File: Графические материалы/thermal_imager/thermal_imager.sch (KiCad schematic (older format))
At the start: 21 parts, among them J1 CONN_in-, J2 CONN_in+, J3 conOut+, J4 conOut-, J5 CONN_bat+, J6 CONN_bat-

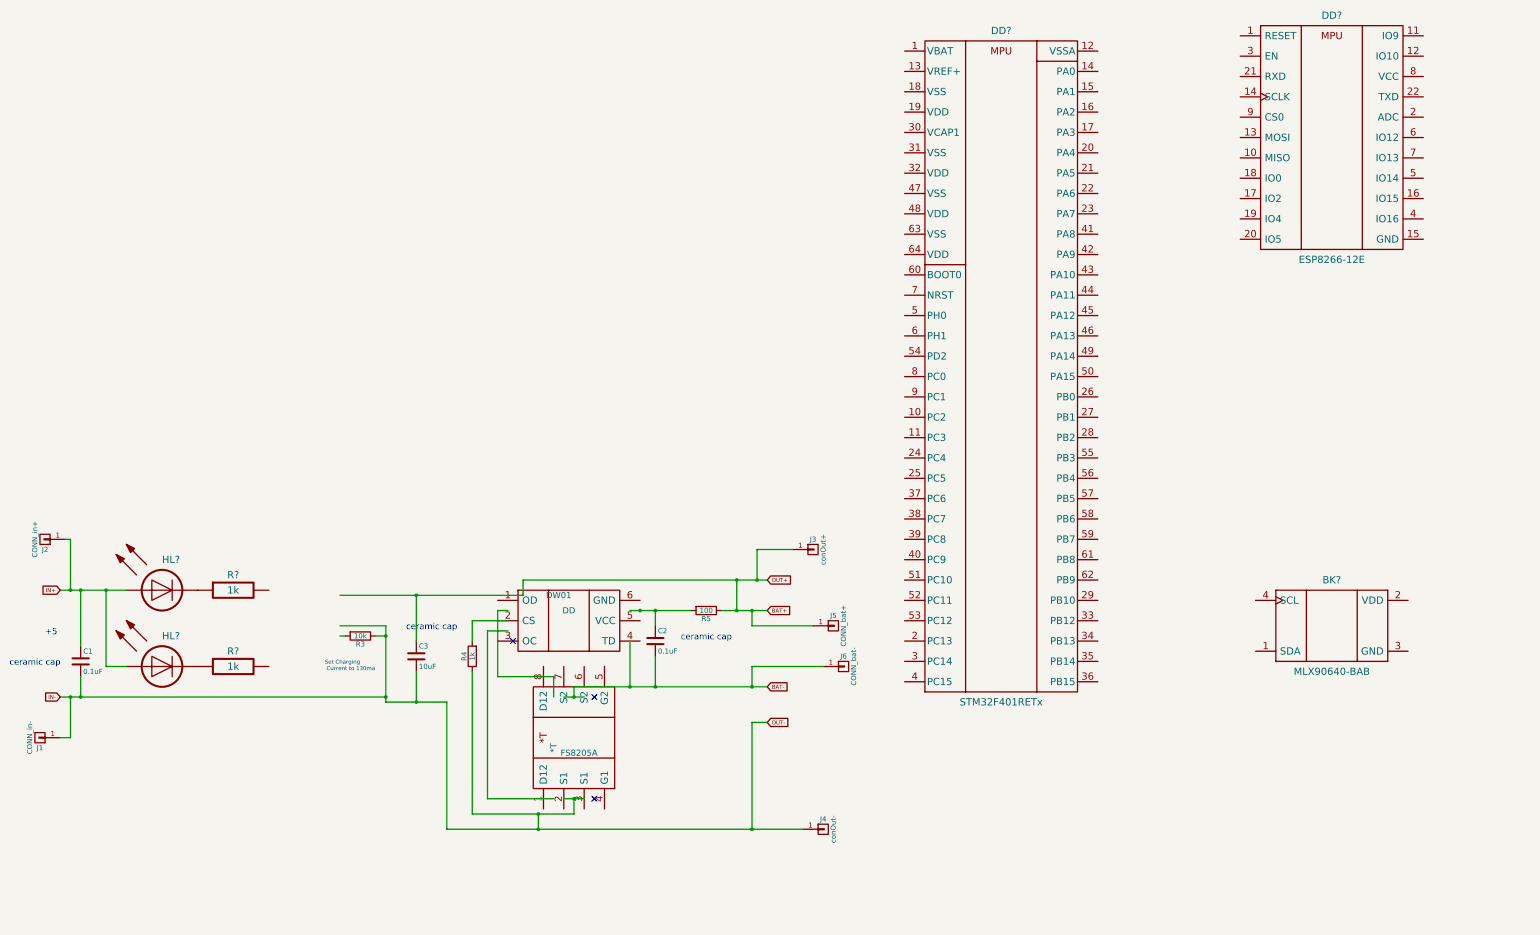
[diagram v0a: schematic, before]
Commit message: Something
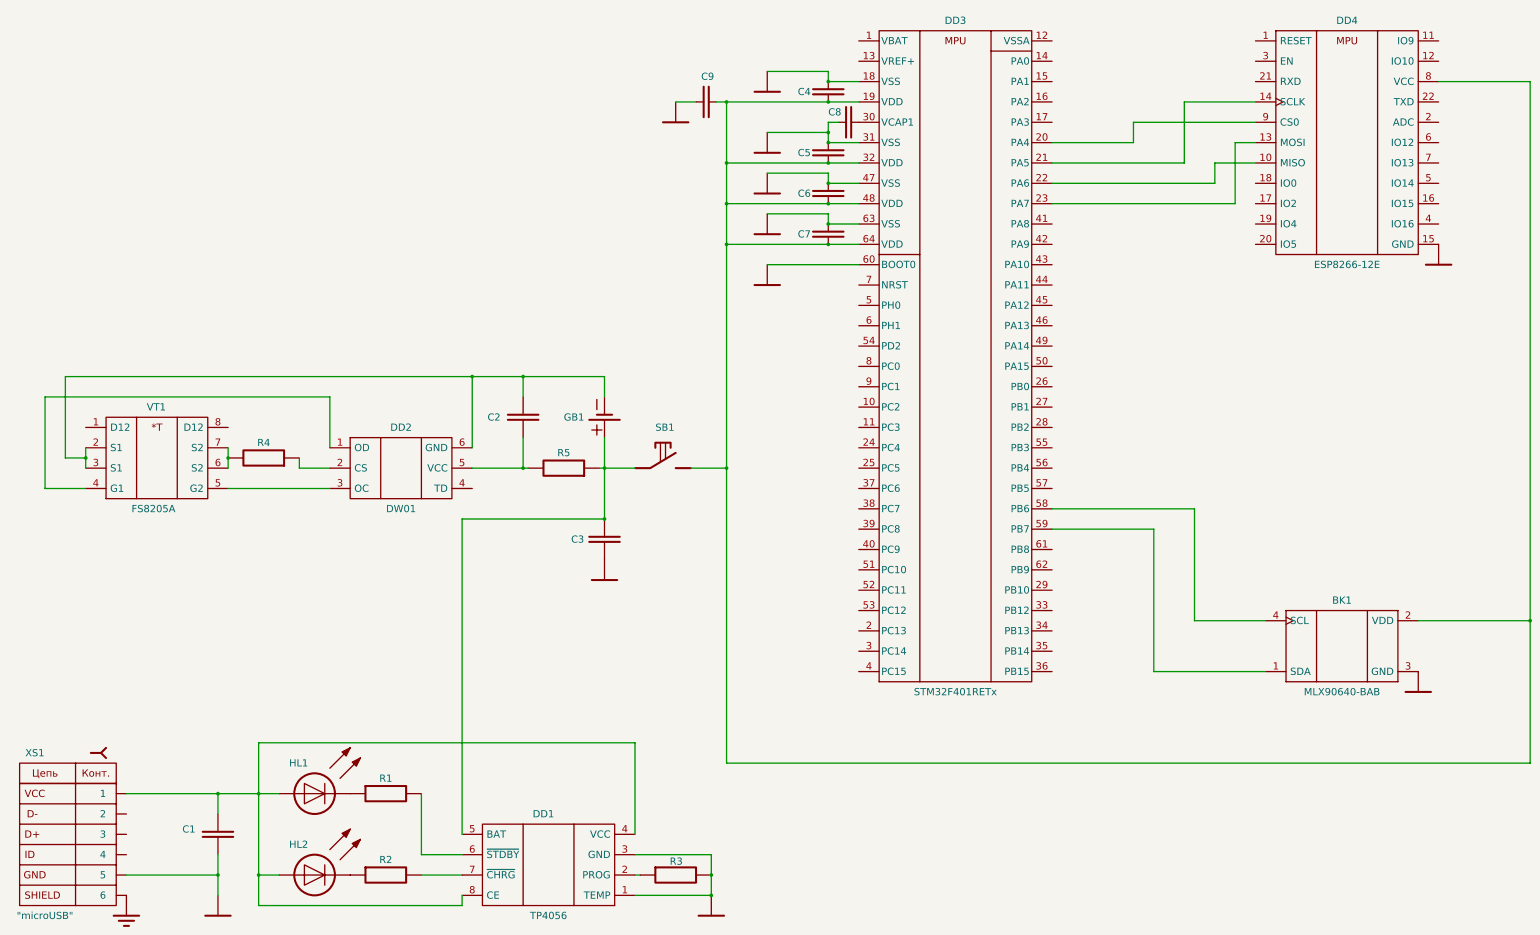
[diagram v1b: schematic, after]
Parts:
- removed *T: FS8205A, Housings_SSOP:TSSOP-8_4.4x3mm_Pitch0.65mm, symbol thermal_imager:FS8205A
- removed C1, C2: 0.1uF, Capacitors_SMD:C_0805_HandSoldering, symbol charger_stepup-rescue:C
- removed C3: 10uF, Capacitors_SMD:C_0805_HandSoldering, symbol charger_stepup-rescue:C
- removed DD: DW01, TO_SOT_Packages_SMD:SOT-23-6_Handsoldering, symbol thermal_imager:DW01
- removed HL? (x2): HL_LED, symbol Diodes:HL_LED
- removed J1: CONN_in-, Pin_Headers:Pin_Header_Straight_1x01_Pitch2.54mm, symbol charger_stepup-rescue:CONN_01X01
- removed J2: CONN_in+, Pin_Headers:Pin_Header_Straight_1x01_Pitch2.54mm, symbol charger_stepup-rescue:CONN_01X01
- removed J3: conOut+, Pin_Headers:Pin_Header_Straight_1x01_Pitch2.54mm, symbol charger_stepup-rescue:CONN_01X01
- removed J4: conOut-, Pin_Headers:Pin_Header_Straight_1x01_Pitch2.54mm, symbol charger_stepup-rescue:CONN_01X01
- removed J5: CONN_bat+, Pin_Headers:Pin_Header_Straight_1x01_Pitch2.54mm, symbol charger_stepup-rescue:CONN_01X01
- removed J6: CONN_bat-, Pin_Headers:Pin_Header_Straight_1x01_Pitch2.54mm, symbol charger_stepup-rescue:CONN_01X01
- removed R3: 10k, Resistors_SMD:R_0603_HandSoldering, symbol charger_stepup-rescue:R
- removed R4: 1k, Resistors_SMD:R_0603_HandSoldering, symbol charger_stepup-rescue:R
- removed R5: 100, Resistors_SMD:R_0603_HandSoldering, symbol charger_stepup-rescue:R
- added C1: 0,1uF, Capacitor_THT:C_Disc_D3.0mm_W1.6mm_P2.50mm, symbol Capacitors:C_CAP
- added C2: 0.1uF, Capacitor_THT:C_Disc_D3.0mm_W1.6mm_P2.50mm, symbol Capacitors:C_CAP
- added C3: 10uF, Capacitor_THT:C_Radial_D4.0mm_H5.0mm_P1.50mm, symbol Capacitors:C_CAP
- added C4, C5, C6, C7: 100nF, Capacitor_THT:C_Disc_D3.0mm_W1.6mm_P2.50mm, symbol thermal_imager:C_CAP
- added C8: 2.2uF, Capacitor_THT:C_Radial_D4.0mm_H5.0mm_P1.50mm, symbol thermal_imager:C_CAP
- added C9: 4.7uF, Capacitor_THT:C_Radial_D4.0mm_H5.0mm_P1.50mm, symbol thermal_imager:C_CAP
- added DD1: TP4056, thermal_imager:SOP-8, symbol thermal_imager:TP4056
- added DD2: DW01, thermal_imager:SOT23-6, symbol thermal_imager:DW01
- added GB1: GB_BATTERY, TestPoint:TestPoint_2Pads_Pitch2.54mm_Drill0.8mm, symbol thermal_imager:GB_BATTERY
- added HL1, HL2: HL_LED, LED_THT:LED_D3.0mm, symbol thermal_imager:HL_LED
- added R3: 10k, Resistor_THT:R_Axial_DIN0204_L3.6mm_D1.6mm_P5.08mm_Horizontal, symbol Resistors:R_RES
- added R4: 1k, Resistor_THT:R_Axial_DIN0204_L3.6mm_D1.6mm_P5.08mm_Horizontal, symbol Resistors:R_RES
- added R5: 100, Resistor_THT:R_Axial_DIN0204_L3.6mm_D1.6mm_P5.08mm_Horizontal, symbol Resistors:R_RES
- added SB1: SB_ON, Button_Switch_THT:SW_DIP_SPSTx01_Slide_6.7x4.1mm_W7.62mm_P2.54mm_LowProfile, symbol Switches:SB_ON
- added VT1: FS8205A, thermal_imager:SOP65P640X120-8N, symbol thermal_imager:FS8205A
- added XS1: \"microUSB\", Connector_USB:USB_Micro-B_Molex-105133-0001, symbol thermal_imager:XS_SOCKET_MICROUSB
- BK1: renamed from BK?; footprint TO292P945H1165-4 -> thermal_imager:TO292P945H1165-4
- DD4: renamed from DD?; footprint XCVR_ESP8266-12E/ESP-12E -> thermal_imager:ESP-12E
- R1, R2: renamed from R?; footprint (none) -> Resistor_THT:R_Axial_DIN0204_L3.6mm_D1.6mm_P5.08mm_Horizontal
- gave numbers to parts that had none: 1
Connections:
- net labels added: GND, GROUND
- net labels removed: BAT+, BAT-, IN+, IN-, OUT+, OUT-
- wire segments 76 -> 105
- no-connect marks 3 -> 0
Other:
- note removed: "+5"
- note removed: "Set Charging\n Current to 130ma\n"
- note removed: "ceramic cap\n"
- moved on the sheet: BK1, DD3, DD4, R1, R2
